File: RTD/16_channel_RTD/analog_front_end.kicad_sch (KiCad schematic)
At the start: 207 parts, among them J1 Screw_Terminal_01x03, J10 Screw_Terminal_01x03, J11 Screw_Terminal_01x03, J12 Screw_Terminal_01x03, J13 Screw_Terminal_01x03, J14 Screw_Terminal_01x03, J15 Screw_Terminal_01x03, J16 Screw_Terminal_01x03, J17 Screw_Terminal_01x03, J2 Screw_Terminal_01x03, J3 Screw_Terminal_01x03, J5 Screw_Terminal_01x03, J6 Screw_Terminal_01x03, J7 Screw_Terminal_01x03, J8 Screw_Terminal_01x03, J9 Screw_Terminal_01x03

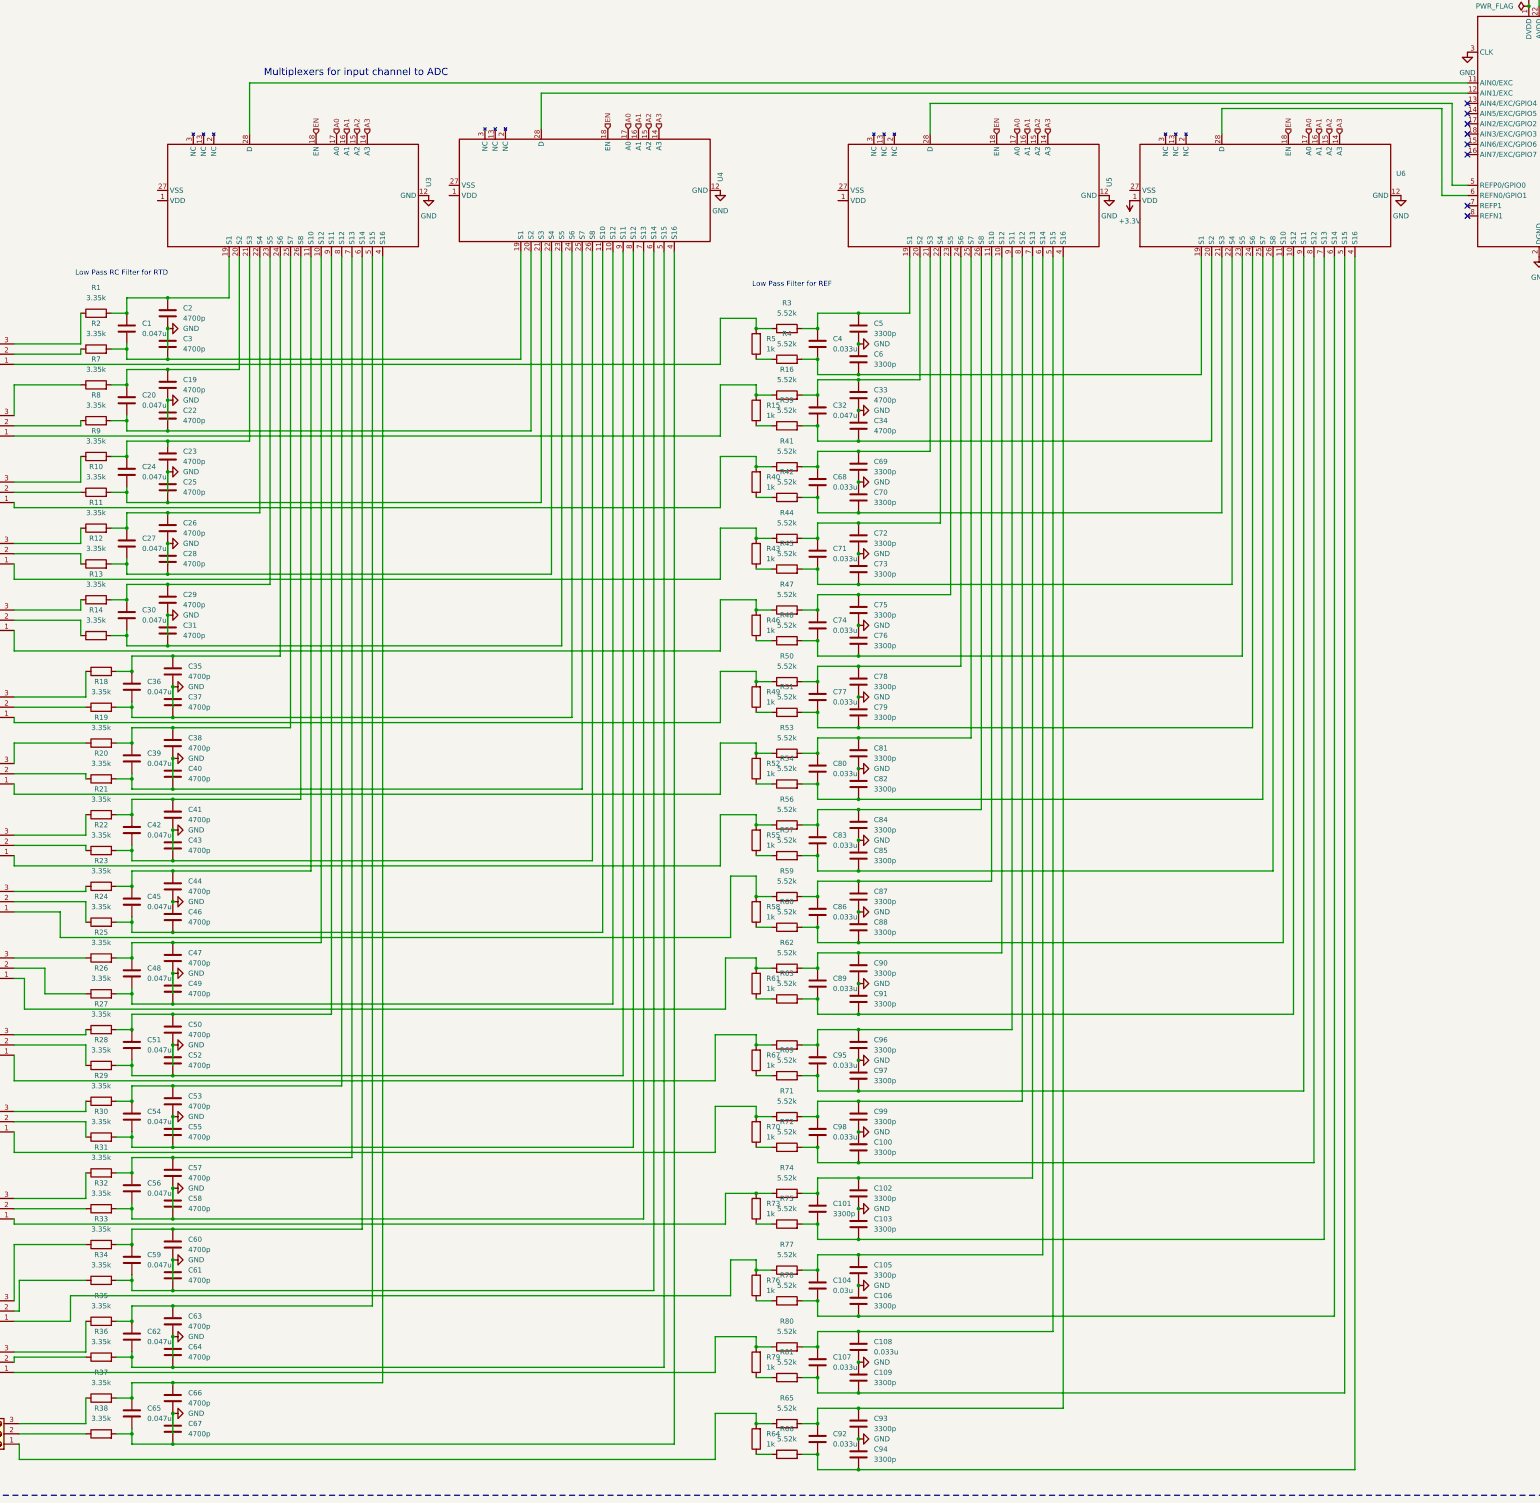
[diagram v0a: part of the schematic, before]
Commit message: ERC free
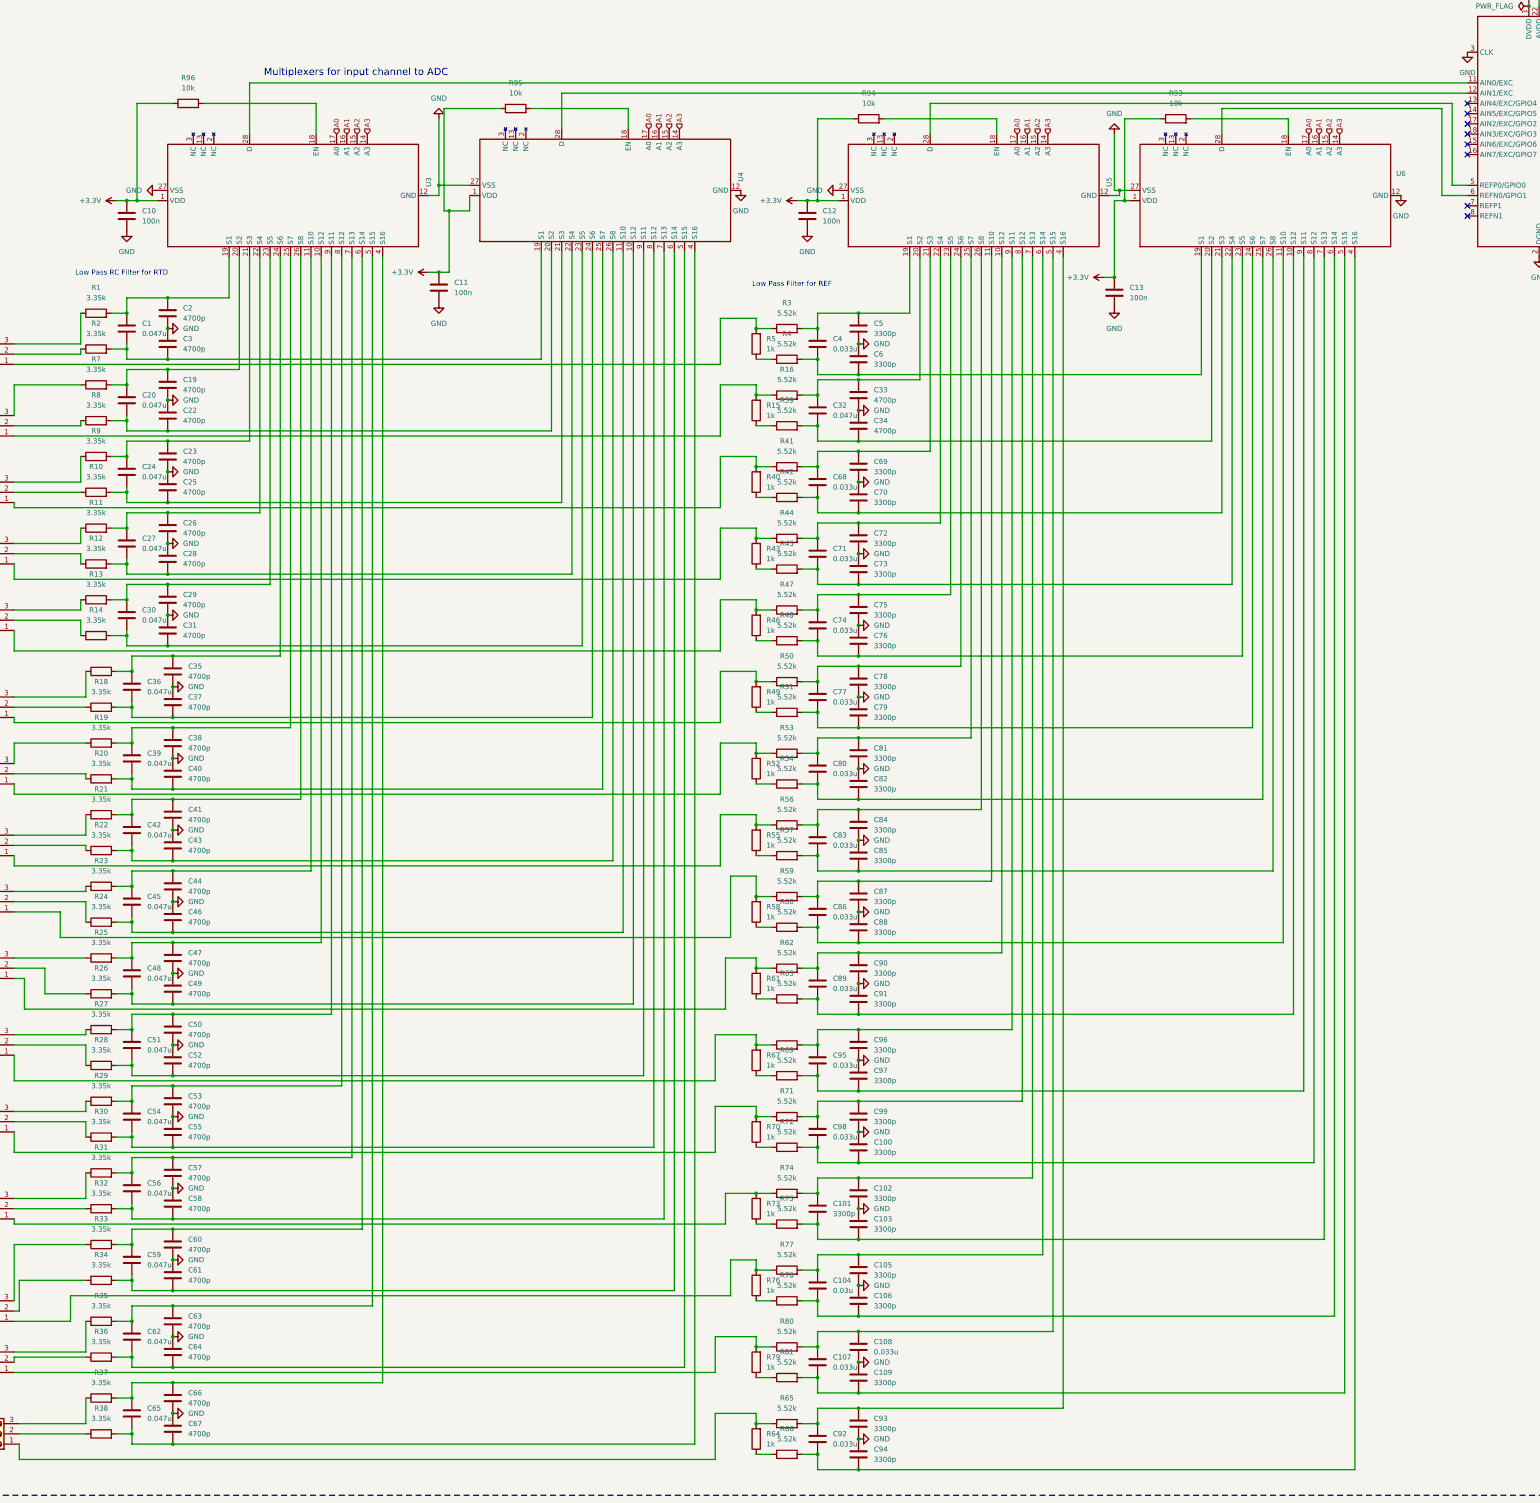
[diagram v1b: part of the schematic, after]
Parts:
- added C10, C11, C12, C13: 100n, symbol Device:C
- added R93, R94, R95, R96: 10k, symbol Device:R
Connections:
- net +3.3V: now also U3.1 (VDD), U4.1 (VDD), U5.1 (VDD), C10.2, C11.2, C12.2, C13.2, R93.1, R94.1, R95.1, R96.1
- net GND: now also U3.27 (VSS), U4.27 (VSS), U5.27 (VSS), U6.27 (VSS), C10.1, C11.1, C12.1, C13.1
- removed net EN: U3.18 (EN), U4.18 (EN), U5.18 (EN), U6.18 (EN)
- new net: R94.2, U5.18 (EN)
- new net: R93.2, U6.18 (EN)
- new net: R95.2, U4.18 (EN)
- new net: R96.2, U3.18 (EN)
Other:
- moved on the sheet: U4
